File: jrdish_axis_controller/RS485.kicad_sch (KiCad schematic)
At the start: 21 parts, among them CN3 KF2EDGR-2.54-4P, CN4 KF2EDGR-2.54-4P, U2 ISOW1432BDFMR

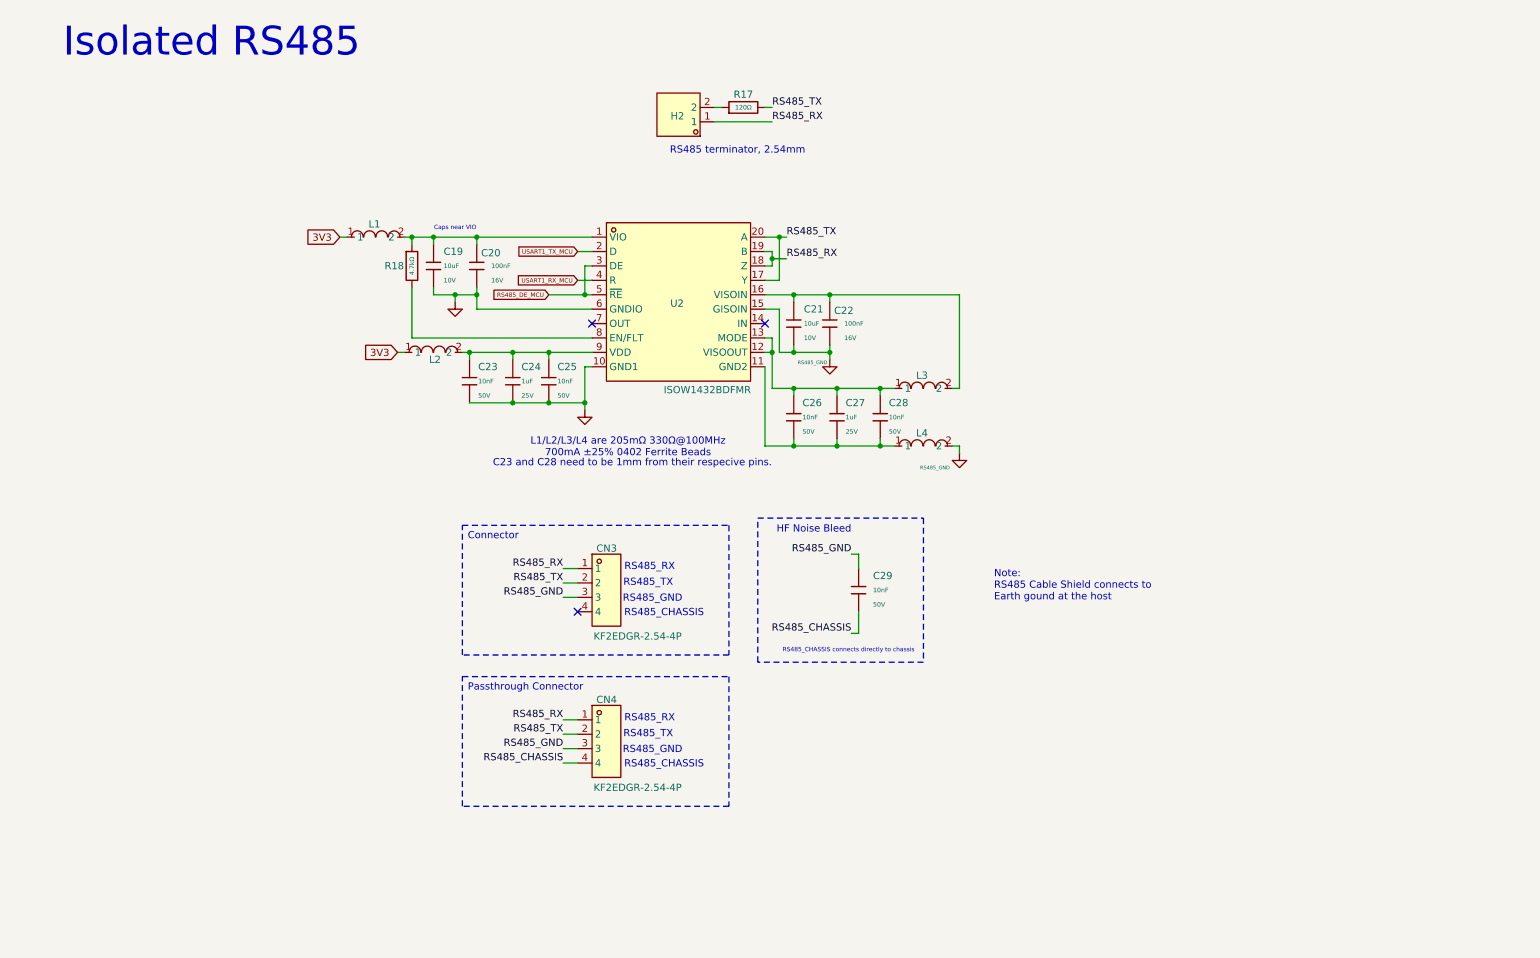
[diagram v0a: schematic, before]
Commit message: Continuing layout
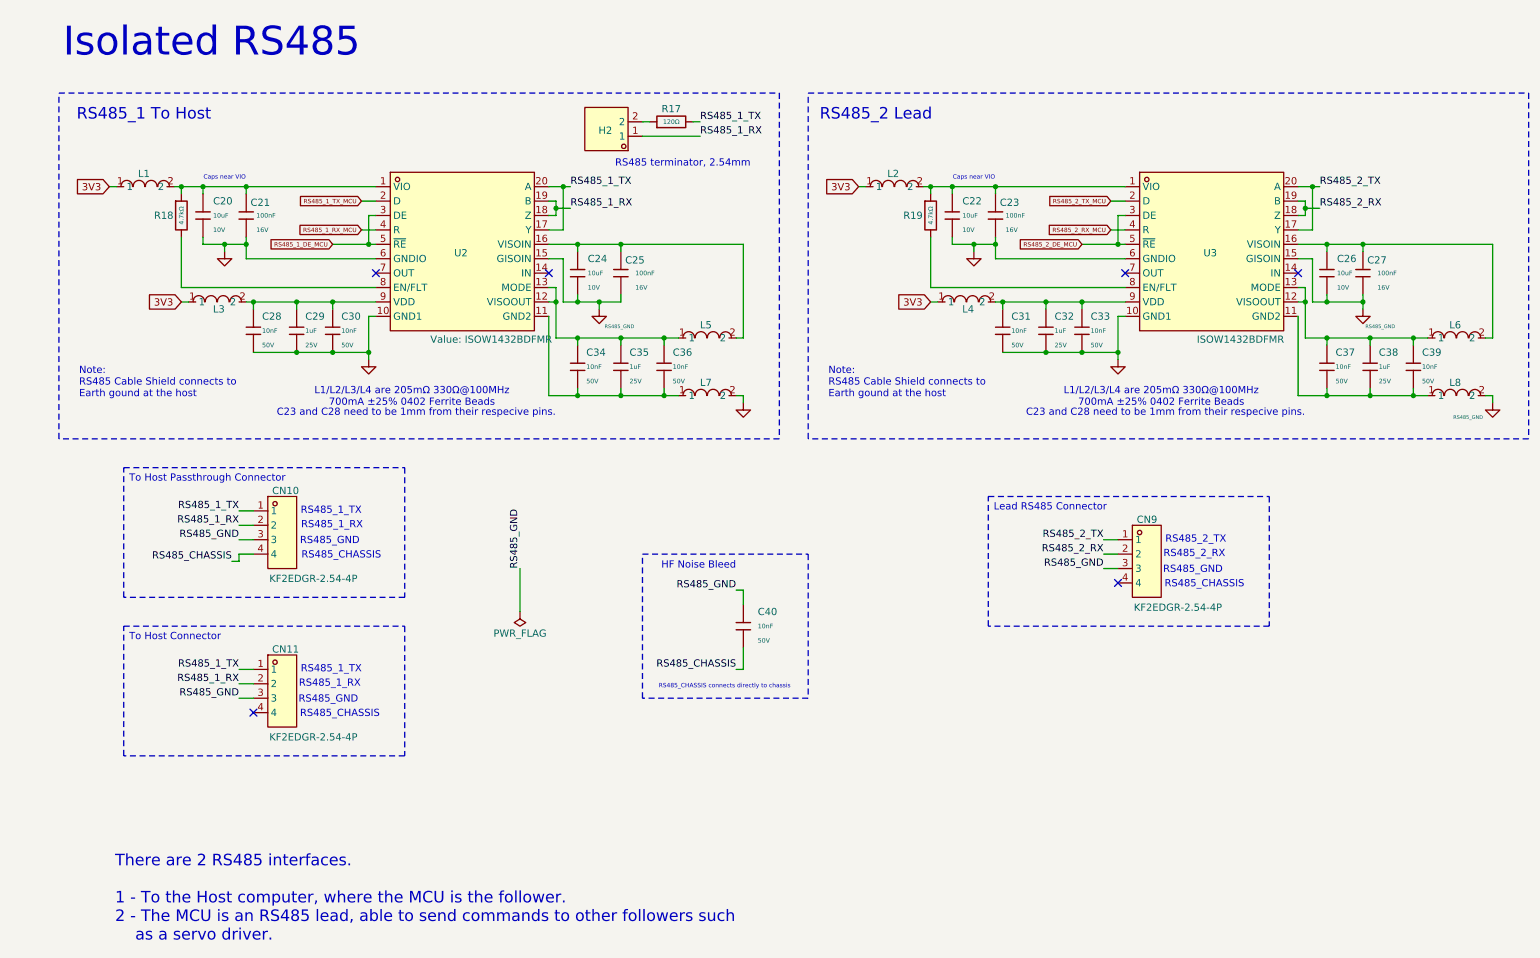
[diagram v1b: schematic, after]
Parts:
- added C22, C26: 10uF, PCM_JLCPCB:C_0603, symbol PCM_JLCPCB-Capacitors:0603,10uF
- added C23, C27: 100nF, PCM_JLCPCB:C_0402, symbol PCM_JLCPCB-Capacitors:0402,100nF
- added C31, C33, C37, C39: 10nF, PCM_JLCPCB:C_0402, symbol PCM_JLCPCB-Capacitors:0402,10nF
- added C32, C38: 1uF, PCM_JLCPCB:C_0402, symbol PCM_JLCPCB-Capacitors:0402,1uF
- added CN9: KF2EDGR-2.54-4P, MyParts:CONN-TH_4P-P2.54_KF2EDGR-2.54-4P, symbol MyParts:KF2EDGR-2.54-4P
- added L2, L4, L6, L8: BLM15EX331SN1D, MyParts:L0402, symbol MyParts:BLM15EX331SN1D
- added R19: 4.7kΩ, PCM_JLCPCB:R_0402, symbol PCM_JLCPCB-Resistors:0402,4.7kΩ
- added U3: ISOW1432BDFMR, MyParts:SOIC-20_L12.8-W7.5-P1.27-LS10.3-BL, symbol MyParts:ISOW1432BDFMR
- renumbered C19 to C20, C20 to C21, C21 to C24, C22 to C25, C23 to C28, C24 to C29, C25 to C30, C26 to C34, C27 to C35, C28 to C36, C29 to C40, CN4 to CN10, CN3 to CN11, L2 to L3, L3 to L5, L4 to L7
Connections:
- net 3V3: now also L2.1, L4.1
- net GND: now also L7.2, C22.2, C23.2, C31.2, C32.2, C33.2, U3.10 (GND1), U3.6 (GNDIO)
- net RS485_GND: now also C26.2, C27.2, CN9.3, L8.2, U3.15 (GISOIN); no longer L7.2
- net RS485_DE_MCU renamed RS485_1_DE_MCU
- net RS485_RX renamed RS485_1_RX
- net RS485_1_RX: now also CN10.2, CN11.2; no longer CN10.1, CN11.1
- net RS485_TX renamed RS485_1_TX
- net RS485_1_TX: now also CN10.1, CN11.1; no longer CN10.2, CN11.2
- net USART1_RX_MCU renamed RS485_1_RX_MCU
- net USART1_TX_MCU renamed RS485_1_TX_MCU
- new net: C37.1, C38.1, C39.1, L6.1, U3.12 (VISOOUT), U3.13 (MODE)
- new net: C26.1, C27.1, L6.2, U3.16 (VISOIN)
- new net: C22.1, C23.1, L2.2, R19.1, U3.1 (VIO)
- new net: C31.1, C32.1, C33.1, L4.2, U3.9 (VDD)
- new net: C37.2, C38.2, C39.2, L8.1, U3.11 (GND2)
- new net: R19.2, U3.8 (EN/FLT)
- new net RS485_2_DE_MCU: U3.3 (DE), U3.5 (~{RE})
- new net RS485_2_RX: CN9.2, U3.18 (Z), U3.19 (B)
- new net RS485_2_RX_MCU: U3.4 (R)
- new net RS485_2_TX: CN9.1, U3.17 (Y), U3.20 (A)
- new net RS485_2_TX_MCU: U3.2 (D)
- no-connect marks 3 -> 6
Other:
- note added: "RS485_1 To Host"
- note added: "RS485_1_RX"
- note added: "RS485_1_TX"
- note added: "RS485_2 Lead"
- note added: "RS485_2_RX"
- note added: "RS485_2_TX"
- note added: "There are 2 RS485 interfaces. 1 - To the Host computer, where the MCU is the follower. 2 - The MCU is an RS485 lead, able to send commands to other followers such as a servo driver."
- note removed: "RS485_RX"
- note removed: "RS485_TX"
- moved on the sheet: C20, C21, C24, C25, C28, C29, C30, C34, C35, C36, C40, CN10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
